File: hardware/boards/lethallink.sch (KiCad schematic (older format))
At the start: 4 parts, among them J1 PCIe-x4

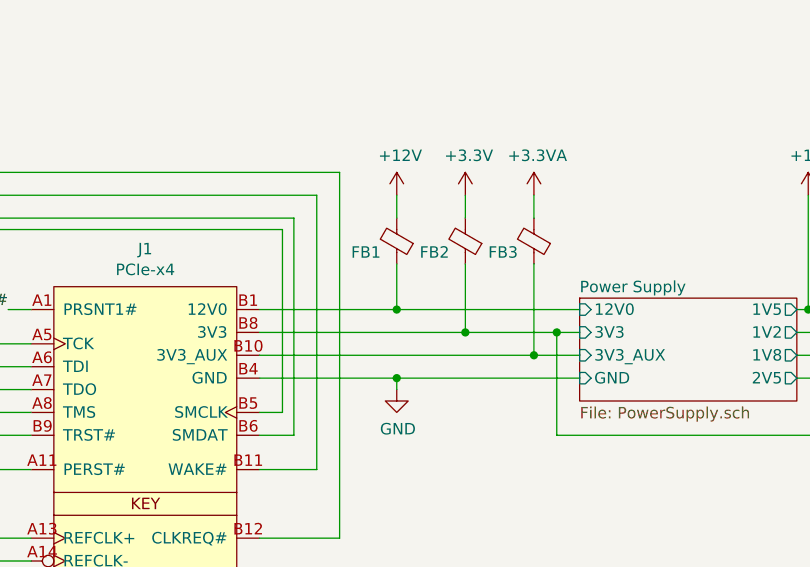
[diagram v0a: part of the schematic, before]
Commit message: Some strugglebusting on getting the ERC errors cleaned up a bit
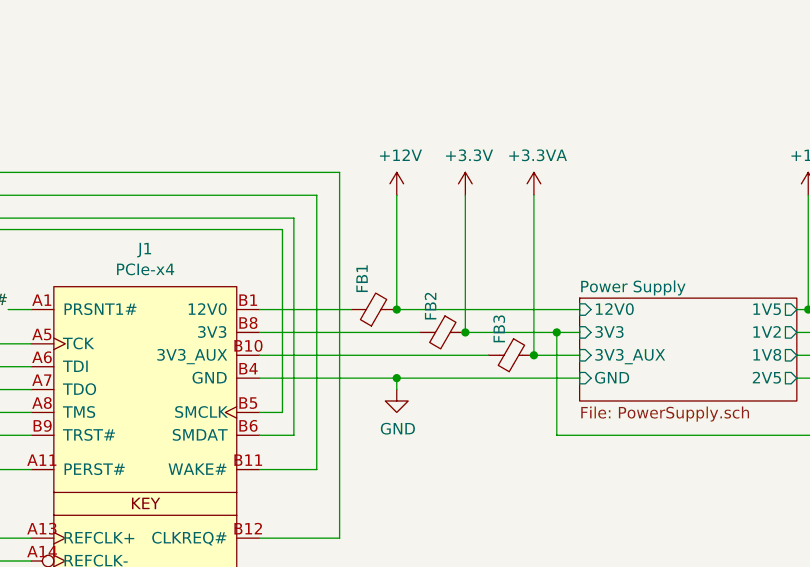
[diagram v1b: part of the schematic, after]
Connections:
- net +3.3VA: now also FB3.1; no longer FB3.2
- net +3V3: now also FB2.1; no longer FB2.2
- net IC Power/3V3: no longer names the net of J1.A10 (3V3), J1.A9 (3V3), J1.B8 (3V3)
- net IC Power/3V3: now also FB2.2; no longer FB2.1
- net Power Supply/12V0: no longer names the net of FB1.1, J1.A2 (12V0), J1.A3 (12V0), J1.B1 (12V0), J1.B2 (12V0), J1.B3 (12V0)
- net Power Supply/3V3_AUX: no longer names the net of J1.B10 (3V3_AUX)
- net Power Supply/3V3_AUX: now also FB3.2; no longer FB3.1
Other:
- moved on the sheet: FB1, FB2, FB3
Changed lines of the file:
@@
 $EndComp
-Wire Wire Line
-	4900 1400 4900 1300
-Wire Wire Line
-	5200 1400 5200 1300
-Wire Wire Line
-	5500 1400 5500 1300
 Wire Wire Line
 	4300 2100 4900 2100
@@
 F9 "1V5" O R 6650 1800 50
 $EndSheet
-Wire Wire Line
-	4300 1800 4900 1800
-Wire Wire Line
-	4300 1900 5200 1900
 $Comp
 L Device:Ferrite_Bead_Small FB1
 U 1 1 5EEA5842
-P 4900 1500
-F 0 "FB1" H 5100 1550 50  0000 R CNN
-F 1 "100 @ 100MHz" H 5050 1700 50  0001 R CNN
-F 2 "Resistor_SMD:R_0603_1608Metric" V 4830 1500 50  0001 C CNN
-F 3 "~" H 4900 1500 50  0001 C CNN
-F 4 "Murata Electronics" H 4900 1500 50  0001 C CNN "MFR"
-F 5 "BLM18KG101TN1D" H 4900 1500 50  0001 C CNN "MPN"
-	1    4900 1500
-	-1   0    0    1
-$EndComp
-Wire Wire Line
-	5500 1600 5500 2000
-Connection ~ 5500 2000
-Wire Wire Line
-	5500 2000 5700 2000
+P 4800 1800
+F 0 "FB1" H 5000 1850 50  0000 R CNN
+F 1 "100 @ 100MHz" H 4950 2000 50  0001 R CNN
+F 2 "Resistor_SMD:R_0603_1608Metric" V 4730 1800 50  0001 C CNN
+F 3 "~" H 4800 1800 50  0001 C CNN
+F 4 "Murata Electronics" H 4800 1800 50  0001 C CNN "MFR"
+F 5 "BLM18KG101TN1D" H 4800 1800 50  0001 C CNN "MPN"
+	1    4800 1800
+	0    -1   -1   0
+$EndComp
 Connection ~ 4900 2100
-Wire Wire Line
-	4900 2100 5700 2100
-Wire Wire Line
-	4300 2000 5500 2000
-Wire Wire Line
-	4900 1600 4900 1800
-Connection ~ 4900 1800
-Wire Wire Line
-	4900 1800 5700 1800
-Wire Wire Line
-	5200 1600 5200 1900
-Connection ~ 5200 1900
-Wire Wire Line
-	5200 1900 5600 1900
 Wire Wire Line
 	6700 1800 7650 1800
@@
 L Device:Ferrite_Bead_Small FB2
 U 1 1 5F579DEB
-P 5200 1500
-F 0 "FB2" H 5400 1550 50  0000 R CNN
-F 1 "220 @ 100Mhz" H 5350 1700 50  0001 R CNN
-F 2 "Resistor_SMD:R_0603_1608Metric" V 5130 1500 50  0001 C CNN
-F 3 "~" H 5200 1500 50  0001 C CNN
-F 4 "Murata Electronics" H 5200 1500 50  0001 C CNN "MFR"
-F 5 "BLM18AG221SN1D" H 5200 1500 50  0001 C CNN "MPN"
-	1    5200 1500
-	-1   0    0    1
+P 5100 1900
+F 0 "FB2" H 5050 1850 50  0000 R CNN
+F 1 "220 @ 100Mhz" H 5250 2100 50  0001 R CNN
+F 2 "Resistor_SMD:R_0603_1608Metric" V 5030 1900 50  0001 C CNN
+F 3 "~" H 5100 1900 50  0001 C CNN
+F 4 "Murata Electronics" H 5100 1900 50  0001 C CNN "MFR"
+F 5 "BLM18AG221SN1D" H 5100 1900 50  0001 C CNN "MPN"
+	1    5100 1900
+	0    1    1    0
 $EndComp
 $Comp
 L Device:Ferrite_Bead_Small FB3
 U 1 1 5F57A174
-P 5500 1500
-F 0 "FB3" H 5700 1550 50  0000 R CNN
-F 1 "220 @ 100Mhz" H 5650 1700 50  0001 R CNN
-F 2 "Resistor_SMD:R_0603_1608Metric" V 5430 1500 50  0001 C CNN
-F 3 "~" H 5500 1500 50  0001 C CNN
-F 4 "Murata Electronics" H 5500 1500 50  0001 C CNN "MFR"
-F 5 "BLM18AG221SN1D" H 5500 1500 50  0001 C CNN "MPN"
-	1    5500 1500
-	-1   0    0    1
+P 5400 2000
+F 0 "FB3" H 5350 1950 50  0000 R CNN
+F 1 "220 @ 100Mhz" H 5550 2200 50  0001 R CNN
+F 2 "Resistor_SMD:R_0603_1608Metric" V 5330 2000 50  0001 C CNN
+F 3 "~" H 5400 2000 50  0001 C CNN
+F 4 "Murata Electronics" H 5400 2000 50  0001 C CNN "MFR"
+F 5 "BLM18AG221SN1D" H 5400 2000 50  0001 C CNN "MPN"
+	1    5400 2000
+	0    1    1    0
 $EndComp
 $Sheet
@@
 F6 "1V5" I L 7650 1800 50
 $EndSheet
+Wire Wire Line
+	4300 1800 4700 1800
+Wire Wire Line
+	4300 1900 5000 1900
+Wire Wire Line
+	5500 2000 5700 2000
+Wire Wire Line
+	4900 1300 4900 1800
+Connection ~ 4900 1800
+Wire Wire Line
+	5200 1300 5200 1900
+Wire Wire Line
+	5500 1300 5500 2000
+Connection ~ 5200 1900
+Wire Wire Line
+	4300 2000 5300 2000
+Wire Wire Line
+	4900 1800 5700 1800
+Connection ~ 5500 2000
+Wire Wire Line
+	4900 2100 5700 2100
+Wire Wire Line
+	5200 1900 5600 1900
 $EndSCHEMATC
